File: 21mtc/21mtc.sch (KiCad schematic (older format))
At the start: 4 parts, among them P101 CONN_01X11, P102 CONN_02X11, P103 CONN_01X11, P104 CONN_02X04

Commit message: Layout of a first draft
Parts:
- removed P101: CONN_01X11, symbol CONN_01X10
- added P101: CONN_01X06, Connectors:solderpads_1x06_2mm, symbol CONN_01X06
- added P105: CONN_01X04, Connectors:solderpads_1x04_2mm, symbol CONN_01X04
- P102: footprint (none) -> Connectors:Pin_Header_Straight_2x11_1.27_smd
- P103: footprint (none) -> Connectors:solderpads_1x11_2mm
- P104: footprint (none) -> Pin_Headers:Pin_Header_Straight_2x04
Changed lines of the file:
@@
 F 0 "P102" H 4650 3800 50  0000 C CNN
 F 1 "CONN_02X11" V 4650 3200 50  0000 C CNN
-F 2 "" H 4650 2000 60  0000 C CNN
+F 2 "Connectors:Pin_Header_Straight_2x11_1.27_smd" H 4650 2000 60  0001 C CNN
 F 3 "" H 4650 2000 60  0000 C CNN
 	1    4650 3200
@@
 F 0 "P103" H 5400 2600 50  0000 C CNN
 F 1 "CONN_01X11" V 5500 3200 50  0000 C CNN
-F 2 "" H 5400 3200 60  0000 C CNN
+F 2 "Connectors:solderpads_1x11_2mm" H 5400 3200 60  0001 C CNN
 F 3 "" H 5400 3200 60  0000 C CNN
 F 4 "Value" H 5400 3200 60  0001 C CNN "Fieldname"
 	1    5400 3200
 	1    0    0    1
-$EndComp
-$Comp
-L CONN_01X10 P101
-U 1 1 566E68DE
-P 3900 3150
-F 0 "P101" H 3900 3700 50  0000 C CNN
-F 1 "CONN_01X11" V 4000 3150 50  0000 C CNN
-F 2 "" H 3900 3150 60  0000 C CNN
-F 3 "" H 3900 3150 60  0000 C CNN
-F 4 "Value" H 3900 3150 60  0001 C CNN "Fieldname"
-	1    3900 3150
-	-1   0    0    -1
 $EndComp
 Wire Wire Line
@@
 F 0 "P104" H 7100 3300 50  0000 C CNN
 F 1 "CONN_02X04" H 7100 2800 50  0000 C CNN
-F 2 "" H 7100 1850 60  0000 C CNN
+F 2 "Pin_Headers:Pin_Header_Straight_2x04" H 7100 1850 60  0001 C CNN
 F 3 "" H 7100 1850 60  0000 C CNN
 	1    7100 3050
@@
 Text Notes 7700 4000 2    60   ~ 0
 NEM 652 / NMRA Medium
+$Comp
+L CONN_01X06 P101
+U 1 1 566EB905
+P 3900 2950
+F 0 "P101" H 3900 3300 50  0000 C CNN
+F 1 "CONN_01X06" V 4000 2950 50  0000 C CNN
+F 2 "Connectors:solderpads_1x06_2mm" H 3900 2950 60  0001 C CNN
+F 3 "" H 3900 2950 60  0000 C CNN
+	1    3900 2950
+	-1   0    0    -1
+$EndComp
+$Comp
+L CONN_01X04 P105
+U 1 1 566EB947
+P 3900 3450
+F 0 "P105" H 3900 3200 50  0000 C CNN
+F 1 "CONN_01X04" V 4000 3450 50  0000 C CNN
+F 2 "Connectors:solderpads_1x04_2mm" H 3900 3450 60  0001 C CNN
+F 3 "" H 3900 3450 60  0000 C CNN
+	1    3900 3450
+	-1   0    0    -1
+$EndComp
 $EndSCHEMATC

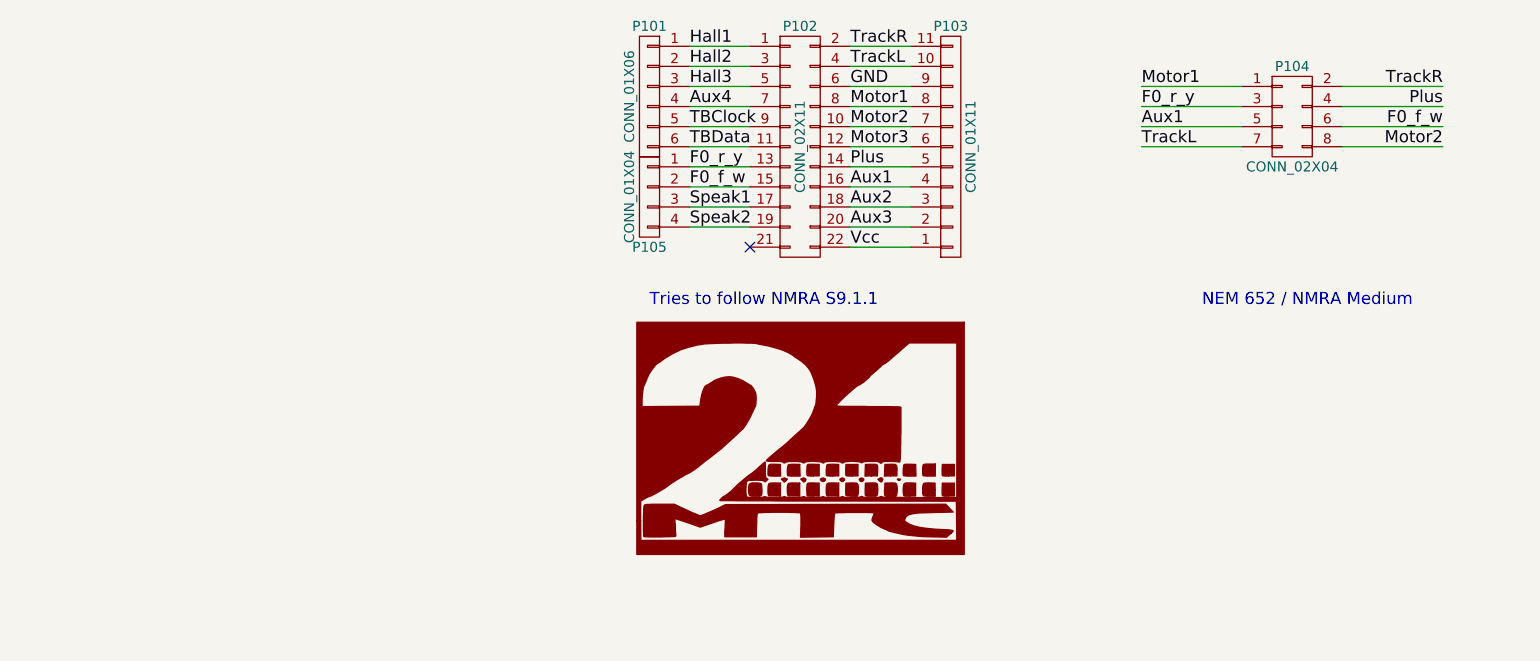
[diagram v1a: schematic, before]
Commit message: MTC21 Updates
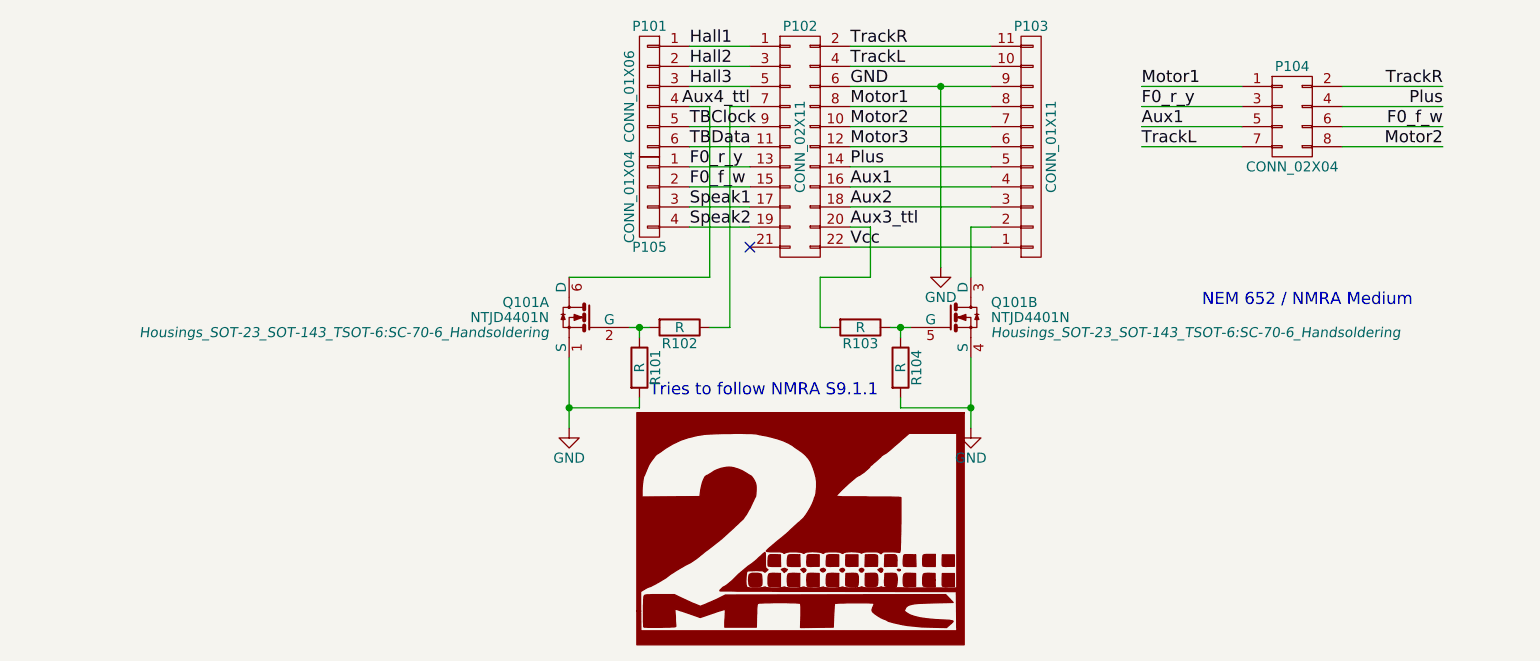
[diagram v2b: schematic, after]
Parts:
- added Q101: NTJD4401N, Housings_SOT-23_SOT-143_TSOT-6:SC-70-6_Handsoldering, symbol NTJD4401N
- added R101, R102, R103, R104: R, Resistors_SMD:R_0805_HandSoldering, symbol R
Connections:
- net GND: now also Q101.1 (S), Q101.4 (S), R101.2, R104.2
- net Aux3: no longer names the net of P103.2 (P2)
- net Aux3: now also Q101.3 (D); no longer P102.20 (P20)
- net Aux4: no longer names the net of P101.4 (P4)
- net Aux4: now also Q101.6 (D); no longer P102.7 (P7)
- new net: Q101.5 (G), R103.1, R104.1
- new net: Q101.2 (G), R101.1, R102.2
- new net Aux3_ttl: P102.20 (P20), R103.2
- new net Aux4_ttl: P102.7 (P7), R102.1
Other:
- moved on the sheet: P103
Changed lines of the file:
@@
 EESchema Schematic File Version 2
+LIBS:21mtc-rescue
 LIBS:power
 LIBS:device
@@
 LIBS:valves
 LIBS:21mtclogo
+LIBS:NTJD4401N
 LIBS:21mtc-cache
 EELAYER 25 0
@@
 L CONN_01X11 P103
 U 1 1 566E68B8
-P 5400 3200
-F 0 "P103" H 5400 2600 50  0000 C CNN
-F 1 "CONN_01X11" V 5500 3200 50  0000 C CNN
-F 2 "Connectors:solderpads_1x11_2mm" H 5400 3200 60  0001 C CNN
-F 3 "" H 5400 3200 60  0000 C CNN
-F 4 "Value" H 5400 3200 60  0001 C CNN "Fieldname"
-	1    5400 3200
+P 5800 3200
+F 0 "P103" H 5800 2600 50  0000 C CNN
+F 1 "CONN_01X11" V 5900 3200 50  0000 C CNN
+F 2 "Connectors:solderpads_1x11_2mm" H 5800 3200 60  0001 C CNN
+F 3 "" H 5800 3200 60  0000 C CNN
+F 4 "Value" H 5800 3200 60  0001 C CNN "Fieldname"
+	1    5800 3200
 	1    0    0    1
 $EndComp
@@
 	4100 2900 4400 2900
 Wire Wire Line
-	4100 3000 4400 3000
-Wire Wire Line
 	4100 3100 4400 3100
 Wire Wire Line
@@
 	4400 3600 4100 3600
 Wire Wire Line
-	4900 2700 5200 2700
-Wire Wire Line
-	5200 2800 4900 2800
-Wire Wire Line
-	4900 2900 5200 2900
-Wire Wire Line
-	5200 3000 4900 3000
-Wire Wire Line
-	4900 3100 5200 3100
-Wire Wire Line
-	4900 3200 5200 3200
-Wire Wire Line
-	5200 3300 4900 3300
-Wire Wire Line
-	4900 3400 5200 3400
-Wire Wire Line
-	5200 3500 4900 3500
-Wire Wire Line
-	4900 3600 5200 3600
-Wire Wire Line
-	5200 3700 4900 3700
+	4900 2700 5600 2700
+Wire Wire Line
+	4900 2800 5600 2800
+Wire Wire Line
+	4900 2900 5600 2900
+Wire Wire Line
+	4900 3000 5600 3000
+Wire Wire Line
+	4900 3100 5600 3100
+Wire Wire Line
+	4900 3200 5600 3200
+Wire Wire Line
+	4900 3300 5600 3300
+Wire Wire Line
+	4900 3400 5600 3400
+Wire Wire Line
+	4900 3500 5600 3500
+Wire Wire Line
+	4900 3700 5600 3700
 Text Label 4100 2700 0    60   ~ 0
 Hall1
@@
 Text Label 4100 2900 0    60   ~ 0
 Hall3
-Text Label 4100 3000 0    60   ~ 0
-Aux4
+Text Label 4400 3000 2    60   ~ 0
+Aux4_ttl
 Text Label 4100 3100 0    60   ~ 0
 TBClock
@@
 Vcc
 Text Label 4900 3600 0    60   ~ 0
-Aux3
+Aux3_ttl
 Text Label 4900 3500 0    60   ~ 0
 Aux2
@@
 L LOGO #G101
 U 1 1 566E6F08
-P 4650 4650
-F 0 "#G101" H 4650 4104 60  0001 C CNN
-F 1 "LOGO" H 4650 5196 60  0001 C CNN
-F 2 "" H 4650 4650 60  0000 C CNN
-F 3 "" H 4650 4650 60  0000 C CNN
-	1    4650 4650
-	1    0    0    -1
-$EndComp
-Text Notes 3900 4000 0    60   ~ 0
+P 4650 5100
+F 0 "#G101" H 4650 4554 60  0001 C CNN
+F 1 "LOGO" H 4650 5646 60  0001 C CNN
+F 2 "" H 4650 5100 60  0000 C CNN
+F 3 "" H 4650 5100 60  0000 C CNN
+	1    4650 5100
+	1    0    0    -1
+$EndComp
+Text Notes 3900 4450 0    60   ~ 0
 Tries to follow NMRA S9.1.1
 $Comp
@@
 	-1   0    0    -1
 $EndComp
+Wire Wire Line
+	4900 3600 5000 3600
+Wire Wire Line
+	4400 3000 4300 3000
+$Comp
+L NTJD4401N Q101
+U 2 1 56717E2C
+P 5400 4050
+F 0 "Q101" H 5600 4125 50  0000 L CNN
+F 1 "NTJD4401N" H 5600 4050 50  0000 L CNN
+F 2 "Housings_SOT-23_SOT-143_TSOT-6:SC-70-6_Handsoldering" H 5600 3975 50  0000 L CIN
+F 3 "" H 5400 4050 50  0000 L CNN
+	2    5400 4050
+	1    0    0    -1
+$EndComp
+$Comp
+L NTJD4401N Q101
+U 1 1 56717E59
+P 3600 4050
+F 0 "Q101" H 3800 4125 50  0000 L CNN
+F 1 "NTJD4401N" H 3800 4050 50  0000 L CNN
+F 2 "Housings_SOT-23_SOT-143_TSOT-6:SC-70-6_Handsoldering" H 3800 3975 50  0000 L CIN
+F 3 "" H 3600 4050 50  0000 L CNN
+	1    3600 4050
+	-1   0    0    -1
+$EndComp
+$Comp
+L R R103
+U 1 1 5673205A
+P 4950 4100
+F 0 "R103" V 5030 4100 50  0000 C CNN
+F 1 "R" V 4950 4100 50  0000 C CNN
+F 2 "Resistors_SMD:R_0805_HandSoldering" V 4880 4100 30  0001 C CNN
+F 3 "" H 4950 4100 30  0000 C CNN
+	1    4950 4100
+	0    1    1    0
+$EndComp
+$Comp
+L R R102
+U 1 1 5673208D
+P 4050 4100
+F 0 "R102" V 4130 4100 50  0000 C CNN
+F 1 "R" V 4050 4100 50  0000 C CNN
+F 2 "Resistors_SMD:R_0805_HandSoldering" V 3980 4100 30  0001 C CNN
+F 3 "" H 4050 4100 30  0000 C CNN
+	1    4050 4100
+	0    1    1    0
+$EndComp
+$Comp
+L R R101
+U 1 1 567320E9
+P 3850 4300
+F 0 "R101" V 3930 4300 50  0000 C CNN
+F 1 "R" V 3850 4300 50  0000 C CNN
+F 2 "Resistors_SMD:R_0805_HandSoldering" V 3780 4300 30  0001 C CNN
+F 3 "" H 3850 4300 30  0000 C CNN
+	1    3850 4300
+	1    0    0    -1
+$EndComp
+$Comp
+L R R104
+U 1 1 5673211C
+P 5150 4300
+F 0 "R104" V 5230 4300 50  0000 C CNN
+F 1 "R" V 5150 4300 50  0000 C CNN
+F 2 "Resistors_SMD:R_0805_HandSoldering" V 5080 4300 30  0001 C CNN
+F 3 "" H 5150 4300 30  0000 C CNN
+	1    5150 4300
+	1    0    0    -1
+$EndComp
+Wire Wire Line
+	5150 4150 5150 4100
+Wire Wire Line
+	5100 4100 5200 4100
+Connection ~ 5150 4100
+Wire Wire Line
+	3900 4100 3800 4100
+Wire Wire Line
+	3850 4150 3850 4100
+Connection ~ 3850 4100
+Wire Wire Line
+	4300 3000 4300 4100
+Wire Wire Line
+	4300 4100 4200 4100
+Wire Wire Line
+	5000 3600 5000 3850
+Wire Wire Line
+	5000 3850 4750 3850
+Wire Wire Line
+	4750 3850 4750 4100
+Wire Wire Line
+	4750 4100 4800 4100
+Wire Wire Line
+	5500 3850 5500 3600
+Wire Wire Line
+	5500 3600 5600 3600
+Wire Wire Line
+	3500 3850 4200 3850
+Wire Wire Line
+	4200 3850 4200 3000
+Wire Wire Line
+	4200 3000 4100 3000
+Wire Wire Line
+	3850 4450 3850 4500
+Wire Wire Line
+	3850 4500 3500 4500
+Wire Wire Line
+	3500 4250 3500 4600
+Wire Wire Line
+	5150 4450 5150 4500
+Wire Wire Line
+	5150 4500 5500 4500
+Wire Wire Line
+	5500 4250 5500 4600
+$Comp
+L GND #PWR01
+U 1 1 5673243C
+P 3500 4600
+F 0 "#PWR01" H 3500 4350 50  0001 C CNN
+F 1 "GND" H 3500 4450 50  0000 C CNN
+F 2 "" H 3500 4600 60  0000 C CNN
+F 3 "" H 3500 4600 60  0000 C CNN
+	1    3500 4600
+	1    0    0    -1
+$EndComp
+$Comp
+L GND #PWR02
+U 1 1 56732471
+P 5500 4600
+F 0 "#PWR02" H 5500 4350 50  0001 C CNN
+F 1 "GND" H 5500 4450 50  0000 C CNN
+F 2 "" H 5500 4600 60  0000 C CNN
+F 3 "" H 5500 4600 60  0000 C CNN
+	1    5500 4600
+	1    0    0    -1
+$EndComp
+$Comp
+L GND #PWR03
+U 1 1 567324A6
+P 5350 3800
+F 0 "#PWR03" H 5350 3550 50  0001 C CNN
+F 1 "GND" H 5350 3650 50  0000 C CNN
+F 2 "" H 5350 3800 60  0000 C CNN
+F 3 "" H 5350 3800 60  0000 C CNN
+	1    5350 3800
+	1    0    0    -1
+$EndComp
+Wire Wire Line
+	5350 3800 5350 2900
+Connection ~ 5350 2900
+Connection ~ 5500 4500
+Connection ~ 3500 4500
 $EndSCHEMATC
